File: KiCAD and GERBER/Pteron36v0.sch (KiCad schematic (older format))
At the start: 56 parts, among them J1 AudioJack4, J2 AudioJack4, J3 Conn_01x04, SW10 SW_PUSH, SW12 SW_PUSH, SW13 SW_PUSH, SW14 SW_PUSH, SW15 SW_PUSH, SW17 SW_PUSH, SW18 SW_PUSH, SW19 SW_PUSH, SW20 SW_PUSH, SW22 SW_PUSH, SW23 SW_PUSH, SW24 SW_PUSH, SW26 SW_PUSH, SW27 SW_PUSH, SW28 SW_PUSH, SW7 SW_PUSH, SW8 SW_PUSH, SW9 SW_PUSH, U1 ProMicro

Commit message: added choc and mx support in single pcb.
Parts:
- SW10, SW12, SW13, SW14, SW15, SW17, SW18, SW19, SW20, SW22, SW23, SW24, SW26, SW27, SW28, SW7, SW8, SW9: footprint Keebio-Parts:Hybrid_PCB_100H_Dual_hole -> Universal-Switch-Footprint:MX-ALPs-PG1350-FLIP
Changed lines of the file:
@@
 F 0 "SW7" H 1550 1755 50  0000 C CNN
 F 1 "SW_PUSH" H 1550 1664 50  0000 C CNN
-F 2 "Keebio-Parts:Hybrid_PCB_100H_Dual_hole" H 1550 1500 60  0001 C CNN
+F 2 "Universal-Switch-Footprint:MX-ALPs-PG1350-FLIP" H 1550 1500 60  0001 C CNN
 F 3 "" H 1550 1500 60  0000 C CNN
 	1    1550 1500
@@
 F 0 "SW8" H 1550 2405 50  0000 C CNN
 F 1 "SW_PUSH" H 1550 2314 50  0000 C CNN
-F 2 "Keebio-Parts:Hybrid_PCB_100H_Dual_hole" H 1550 2150 60  0001 C CNN
+F 2 "Universal-Switch-Footprint:MX-ALPs-PG1350-FLIP" H 1550 2150 60  0001 C CNN
 F 3 "" H 1550 2150 60  0000 C CNN
 	1    1550 2150
@@
 F 0 "SW9" H 1550 3005 50  0000 C CNN
 F 1 "SW_PUSH" H 1550 2914 50  0000 C CNN
-F 2 "Keebio-Parts:Hybrid_PCB_100H_Dual_hole" H 1550 2750 60  0001 C CNN
+F 2 "Universal-Switch-Footprint:MX-ALPs-PG1350-FLIP" H 1550 2750 60  0001 C CNN
 F 3 "" H 1550 2750 60  0000 C CNN
 	1    1550 2750
@@
 F 0 "SW12" H 2200 1755 50  0000 C CNN
 F 1 "SW_PUSH" H 2200 1664 50  0000 C CNN
-F 2 "Keebio-Parts:Hybrid_PCB_100H_Dual_hole" H 2200 1500 60  0001 C CNN
+F 2 "Universal-Switch-Footprint:MX-ALPs-PG1350-FLIP" H 2200 1500 60  0001 C CNN
 F 3 "" H 2200 1500 60  0000 C CNN
 	1    2200 1500
@@
 F 0 "SW13" H 2200 2405 50  0000 C CNN
 F 1 "SW_PUSH" H 2200 2314 50  0000 C CNN
-F 2 "Keebio-Parts:Hybrid_PCB_100H_Dual_hole" H 2200 2150 60  0001 C CNN
+F 2 "Universal-Switch-Footprint:MX-ALPs-PG1350-FLIP" H 2200 2150 60  0001 C CNN
 F 3 "" H 2200 2150 60  0000 C CNN
 	1    2200 2150
@@
 F 0 "SW14" H 2200 3005 50  0000 C CNN
 F 1 "SW_PUSH" H 2200 2914 50  0000 C CNN
-F 2 "Keebio-Parts:Hybrid_PCB_100H_Dual_hole" H 2200 2750 60  0001 C CNN
+F 2 "Universal-Switch-Footprint:MX-ALPs-PG1350-FLIP" H 2200 2750 60  0001 C CNN
 F 3 "" H 2200 2750 60  0000 C CNN
 	1    2200 2750
@@
 F 0 "SW17" H 2850 1755 50  0000 C CNN
 F 1 "SW_PUSH" H 2850 1664 50  0000 C CNN
-F 2 "Keebio-Parts:Hybrid_PCB_100H_Dual_hole" H 2850 1500 60  0001 C CNN
+F 2 "Universal-Switch-Footprint:MX-ALPs-PG1350-FLIP" H 2850 1500 60  0001 C CNN
 F 3 "" H 2850 1500 60  0000 C CNN
 	1    2850 1500
@@
 F 0 "SW22" H 3500 1755 50  0000 C CNN
 F 1 "SW_PUSH" H 3500 1664 50  0000 C CNN
-F 2 "Keebio-Parts:Hybrid_PCB_100H_Dual_hole" H 3500 1500 60  0001 C CNN
+F 2 "Universal-Switch-Footprint:MX-ALPs-PG1350-FLIP" H 3500 1500 60  0001 C CNN
 F 3 "" H 3500 1500 60  0000 C CNN
 	1    3500 1500
@@
 F 0 "SW18" H 2850 2405 50  0000 C CNN
 F 1 "SW_PUSH" H 2850 2314 50  0000 C CNN
-F 2 "Keebio-Parts:Hybrid_PCB_100H_Dual_hole" H 2850 2150 60  0001 C CNN
+F 2 "Universal-Switch-Footprint:MX-ALPs-PG1350-FLIP" H 2850 2150 60  0001 C CNN
 F 3 "" H 2850 2150 60  0000 C CNN
 	1    2850 2150
@@
 F 0 "SW19" H 2850 3005 50  0000 C CNN
 F 1 "SW_PUSH" H 2850 2914 50  0000 C CNN
-F 2 "Keebio-Parts:Hybrid_PCB_100H_Dual_hole" H 2850 2750 60  0001 C CNN
+F 2 "Universal-Switch-Footprint:MX-ALPs-PG1350-FLIP" H 2850 2750 60  0001 C CNN
 F 3 "" H 2850 2750 60  0000 C CNN
 	1    2850 2750
@@
 F 0 "SW23" H 3500 2405 50  0000 C CNN
 F 1 "SW_PUSH" H 3500 2314 50  0000 C CNN
-F 2 "Keebio-Parts:Hybrid_PCB_100H_Dual_hole" H 3500 2150 60  0001 C CNN
+F 2 "Universal-Switch-Footprint:MX-ALPs-PG1350-FLIP" H 3500 2150 60  0001 C CNN
 F 3 "" H 3500 2150 60  0000 C CNN
 	1    3500 2150
@@
 F 0 "SW24" H 3500 3005 50  0000 C CNN
 F 1 "SW_PUSH" H 3500 2914 50  0000 C CNN
-F 2 "Keebio-Parts:Hybrid_PCB_100H_Dual_hole" H 3500 2750 60  0001 C CNN
+F 2 "Universal-Switch-Footprint:MX-ALPs-PG1350-FLIP" H 3500 2750 60  0001 C CNN
 F 3 "" H 3500 2750 60  0000 C CNN
 	1    3500 2750
@@
 F 0 "SW26" H 4150 1755 50  0000 C CNN
 F 1 "SW_PUSH" H 4150 1664 50  0000 C CNN
-F 2 "Keebio-Parts:Hybrid_PCB_100H_Dual_hole" H 4150 1500 60  0001 C CNN
+F 2 "Universal-Switch-Footprint:MX-ALPs-PG1350-FLIP" H 4150 1500 60  0001 C CNN
 F 3 "" H 4150 1500 60  0000 C CNN
 	1    4150 1500
@@
 F 0 "SW27" H 4150 2405 50  0000 C CNN
 F 1 "SW_PUSH" H 4150 2314 50  0000 C CNN
-F 2 "Keebio-Parts:Hybrid_PCB_100H_Dual_hole" H 4150 2150 60  0001 C CNN
+F 2 "Universal-Switch-Footprint:MX-ALPs-PG1350-FLIP" H 4150 2150 60  0001 C CNN
 F 3 "" H 4150 2150 60  0000 C CNN
 	1    4150 2150
@@
 F 0 "SW28" H 4150 3005 50  0000 C CNN
 F 1 "SW_PUSH" H 4150 2914 50  0000 C CNN
-F 2 "Keebio-Parts:Hybrid_PCB_100H_Dual_hole" H 4150 2750 60  0001 C CNN
+F 2 "Universal-Switch-Footprint:MX-ALPs-PG1350-FLIP" H 4150 2750 60  0001 C CNN
 F 3 "" H 4150 2750 60  0000 C CNN
 	1    4150 2750
@@
 F 0 "SW10" H 1550 3605 50  0000 C CNN
 F 1 "SW_PUSH" H 1550 3514 50  0000 C CNN
-F 2 "Keebio-Parts:Hybrid_PCB_100H_Dual_hole" H 1550 3350 60  0001 C CNN
+F 2 "Universal-Switch-Footprint:MX-ALPs-PG1350-FLIP" H 1550 3350 60  0001 C CNN
 F 3 "" H 1550 3350 60  0000 C CNN
 	1    1550 3350
@@
 F 0 "SW15" H 2200 3605 50  0000 C CNN
 F 1 "SW_PUSH" H 2200 3514 50  0000 C CNN
-F 2 "Keebio-Parts:Hybrid_PCB_100H_Dual_hole" H 2200 3350 60  0001 C CNN
+F 2 "Universal-Switch-Footprint:MX-ALPs-PG1350-FLIP" H 2200 3350 60  0001 C CNN
 F 3 "" H 2200 3350 60  0000 C CNN
 	1    2200 3350
@@
 F 0 "SW20" H 2850 3605 50  0000 C CNN
 F 1 "SW_PUSH" H 2850 3514 50  0000 C CNN
-F 2 "Keebio-Parts:Hybrid_PCB_100H_Dual_hole" H 2850 3350 60  0001 C CNN
+F 2 "Universal-Switch-Footprint:MX-ALPs-PG1350-FLIP" H 2850 3350 60  0001 C CNN
 F 3 "" H 2850 3350 60  0000 C CNN
 	1    2850 3350

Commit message: merge version 1.2.0 pcb into main
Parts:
- SW10, SW12, SW13, SW14, SW15, SW17, SW18, SW19, SW20, SW22, SW23, SW24, SW26, SW27, SW28, SW7, SW8, SW9: footprint Universal-Switch-Footprint:MX-ALPs-PG1350-FLIP -> Universal-Switch-Footprint:MX-ALPs-PG1350-FLIP-fix
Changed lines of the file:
@@
 F 0 "SW7" H 1550 1755 50  0000 C CNN
 F 1 "SW_PUSH" H 1550 1664 50  0000 C CNN
-F 2 "Universal-Switch-Footprint:MX-ALPs-PG1350-FLIP" H 1550 1500 60  0001 C CNN
+F 2 "Universal-Switch-Footprint:MX-ALPs-PG1350-FLIP-fix" H 1550 1500 60  0001 C CNN
 F 3 "" H 1550 1500 60  0000 C CNN
 	1    1550 1500
@@
 F 0 "SW8" H 1550 2405 50  0000 C CNN
 F 1 "SW_PUSH" H 1550 2314 50  0000 C CNN
-F 2 "Universal-Switch-Footprint:MX-ALPs-PG1350-FLIP" H 1550 2150 60  0001 C CNN
+F 2 "Universal-Switch-Footprint:MX-ALPs-PG1350-FLIP-fix" H 1550 2150 60  0001 C CNN
 F 3 "" H 1550 2150 60  0000 C CNN
 	1    1550 2150
@@
 F 0 "SW9" H 1550 3005 50  0000 C CNN
 F 1 "SW_PUSH" H 1550 2914 50  0000 C CNN
-F 2 "Universal-Switch-Footprint:MX-ALPs-PG1350-FLIP" H 1550 2750 60  0001 C CNN
+F 2 "Universal-Switch-Footprint:MX-ALPs-PG1350-FLIP-fix" H 1550 2750 60  0001 C CNN
 F 3 "" H 1550 2750 60  0000 C CNN
 	1    1550 2750
@@
 F 0 "SW12" H 2200 1755 50  0000 C CNN
 F 1 "SW_PUSH" H 2200 1664 50  0000 C CNN
-F 2 "Universal-Switch-Footprint:MX-ALPs-PG1350-FLIP" H 2200 1500 60  0001 C CNN
+F 2 "Universal-Switch-Footprint:MX-ALPs-PG1350-FLIP-fix" H 2200 1500 60  0001 C CNN
 F 3 "" H 2200 1500 60  0000 C CNN
 	1    2200 1500
@@
 F 0 "SW13" H 2200 2405 50  0000 C CNN
 F 1 "SW_PUSH" H 2200 2314 50  0000 C CNN
-F 2 "Universal-Switch-Footprint:MX-ALPs-PG1350-FLIP" H 2200 2150 60  0001 C CNN
+F 2 "Universal-Switch-Footprint:MX-ALPs-PG1350-FLIP-fix" H 2200 2150 60  0001 C CNN
 F 3 "" H 2200 2150 60  0000 C CNN
 	1    2200 2150
@@
 F 0 "SW14" H 2200 3005 50  0000 C CNN
 F 1 "SW_PUSH" H 2200 2914 50  0000 C CNN
-F 2 "Universal-Switch-Footprint:MX-ALPs-PG1350-FLIP" H 2200 2750 60  0001 C CNN
+F 2 "Universal-Switch-Footprint:MX-ALPs-PG1350-FLIP-fix" H 2200 2750 60  0001 C CNN
 F 3 "" H 2200 2750 60  0000 C CNN
 	1    2200 2750
@@
 F 0 "SW17" H 2850 1755 50  0000 C CNN
 F 1 "SW_PUSH" H 2850 1664 50  0000 C CNN
-F 2 "Universal-Switch-Footprint:MX-ALPs-PG1350-FLIP" H 2850 1500 60  0001 C CNN
+F 2 "Universal-Switch-Footprint:MX-ALPs-PG1350-FLIP-fix" H 2850 1500 60  0001 C CNN
 F 3 "" H 2850 1500 60  0000 C CNN
 	1    2850 1500
@@
 F 0 "SW22" H 3500 1755 50  0000 C CNN
 F 1 "SW_PUSH" H 3500 1664 50  0000 C CNN
-F 2 "Universal-Switch-Footprint:MX-ALPs-PG1350-FLIP" H 3500 1500 60  0001 C CNN
+F 2 "Universal-Switch-Footprint:MX-ALPs-PG1350-FLIP-fix" H 3500 1500 60  0001 C CNN
 F 3 "" H 3500 1500 60  0000 C CNN
 	1    3500 1500
@@
 F 0 "SW18" H 2850 2405 50  0000 C CNN
 F 1 "SW_PUSH" H 2850 2314 50  0000 C CNN
-F 2 "Universal-Switch-Footprint:MX-ALPs-PG1350-FLIP" H 2850 2150 60  0001 C CNN
+F 2 "Universal-Switch-Footprint:MX-ALPs-PG1350-FLIP-fix" H 2850 2150 60  0001 C CNN
 F 3 "" H 2850 2150 60  0000 C CNN
 	1    2850 2150
@@
 F 0 "SW19" H 2850 3005 50  0000 C CNN
 F 1 "SW_PUSH" H 2850 2914 50  0000 C CNN
-F 2 "Universal-Switch-Footprint:MX-ALPs-PG1350-FLIP" H 2850 2750 60  0001 C CNN
+F 2 "Universal-Switch-Footprint:MX-ALPs-PG1350-FLIP-fix" H 2850 2750 60  0001 C CNN
 F 3 "" H 2850 2750 60  0000 C CNN
 	1    2850 2750
@@
 F 0 "SW23" H 3500 2405 50  0000 C CNN
 F 1 "SW_PUSH" H 3500 2314 50  0000 C CNN
-F 2 "Universal-Switch-Footprint:MX-ALPs-PG1350-FLIP" H 3500 2150 60  0001 C CNN
+F 2 "Universal-Switch-Footprint:MX-ALPs-PG1350-FLIP-fix" H 3500 2150 60  0001 C CNN
 F 3 "" H 3500 2150 60  0000 C CNN
 	1    3500 2150
@@
 F 0 "SW24" H 3500 3005 50  0000 C CNN
 F 1 "SW_PUSH" H 3500 2914 50  0000 C CNN
-F 2 "Universal-Switch-Footprint:MX-ALPs-PG1350-FLIP" H 3500 2750 60  0001 C CNN
+F 2 "Universal-Switch-Footprint:MX-ALPs-PG1350-FLIP-fix" H 3500 2750 60  0001 C CNN
 F 3 "" H 3500 2750 60  0000 C CNN
 	1    3500 2750
@@
 F 0 "SW26" H 4150 1755 50  0000 C CNN
 F 1 "SW_PUSH" H 4150 1664 50  0000 C CNN
-F 2 "Universal-Switch-Footprint:MX-ALPs-PG1350-FLIP" H 4150 1500 60  0001 C CNN
+F 2 "Universal-Switch-Footprint:MX-ALPs-PG1350-FLIP-fix" H 4150 1500 60  0001 C CNN
 F 3 "" H 4150 1500 60  0000 C CNN
 	1    4150 1500
@@
 F 0 "SW27" H 4150 2405 50  0000 C CNN
 F 1 "SW_PUSH" H 4150 2314 50  0000 C CNN
-F 2 "Universal-Switch-Footprint:MX-ALPs-PG1350-FLIP" H 4150 2150 60  0001 C CNN
+F 2 "Universal-Switch-Footprint:MX-ALPs-PG1350-FLIP-fix" H 4150 2150 60  0001 C CNN
 F 3 "" H 4150 2150 60  0000 C CNN
 	1    4150 2150
@@
 F 0 "SW28" H 4150 3005 50  0000 C CNN
 F 1 "SW_PUSH" H 4150 2914 50  0000 C CNN
-F 2 "Universal-Switch-Footprint:MX-ALPs-PG1350-FLIP" H 4150 2750 60  0001 C CNN
+F 2 "Universal-Switch-Footprint:MX-ALPs-PG1350-FLIP-fix" H 4150 2750 60  0001 C CNN
 F 3 "" H 4150 2750 60  0000 C CNN
 	1    4150 2750
@@
 F 0 "SW10" H 1550 3605 50  0000 C CNN
 F 1 "SW_PUSH" H 1550 3514 50  0000 C CNN
-F 2 "Universal-Switch-Footprint:MX-ALPs-PG1350-FLIP" H 1550 3350 60  0001 C CNN
+F 2 "Universal-Switch-Footprint:MX-ALPs-PG1350-FLIP-fix" H 1550 3350 60  0001 C CNN
 F 3 "" H 1550 3350 60  0000 C CNN
 	1    1550 3350
@@
 F 0 "SW15" H 2200 3605 50  0000 C CNN
 F 1 "SW_PUSH" H 2200 3514 50  0000 C CNN
-F 2 "Universal-Switch-Footprint:MX-ALPs-PG1350-FLIP" H 2200 3350 60  0001 C CNN
+F 2 "Universal-Switch-Footprint:MX-ALPs-PG1350-FLIP-fix" H 2200 3350 60  0001 C CNN
 F 3 "" H 2200 3350 60  0000 C CNN
 	1    2200 3350
@@
 F 0 "SW20" H 2850 3605 50  0000 C CNN
 F 1 "SW_PUSH" H 2850 3514 50  0000 C CNN
-F 2 "Universal-Switch-Footprint:MX-ALPs-PG1350-FLIP" H 2850 3350 60  0001 C CNN
+F 2 "Universal-Switch-Footprint:MX-ALPs-PG1350-FLIP-fix" H 2850 3350 60  0001 C CNN
 F 3 "" H 2850 3350 60  0000 C CNN
 	1    2850 3350

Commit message: use crkbd footprint for better manufacturing
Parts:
- SW10, SW12, SW13, SW14, SW15, SW17, SW18, SW19, SW20, SW22, SW23, SW24, SW26, SW27, SW28, SW7, SW8, SW9: footprint Universal-Switch-Footprint:MX-ALPs-PG1350-FLIP-fix -> User-Submitted:uni-new
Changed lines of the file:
@@
 F 0 "SW7" H 1550 1755 50  0000 C CNN
 F 1 "SW_PUSH" H 1550 1664 50  0000 C CNN
-F 2 "Universal-Switch-Footprint:MX-ALPs-PG1350-FLIP-fix" H 1550 1500 60  0001 C CNN
+F 2 "User-Submitted:uni-new" H 1550 1500 60  0001 C CNN
 F 3 "" H 1550 1500 60  0000 C CNN
 	1    1550 1500
@@
 F 0 "SW8" H 1550 2405 50  0000 C CNN
 F 1 "SW_PUSH" H 1550 2314 50  0000 C CNN
-F 2 "Universal-Switch-Footprint:MX-ALPs-PG1350-FLIP-fix" H 1550 2150 60  0001 C CNN
+F 2 "User-Submitted:uni-new" H 1550 2150 60  0001 C CNN
 F 3 "" H 1550 2150 60  0000 C CNN
 	1    1550 2150
@@
 F 0 "SW9" H 1550 3005 50  0000 C CNN
 F 1 "SW_PUSH" H 1550 2914 50  0000 C CNN
-F 2 "Universal-Switch-Footprint:MX-ALPs-PG1350-FLIP-fix" H 1550 2750 60  0001 C CNN
+F 2 "User-Submitted:uni-new" H 1550 2750 60  0001 C CNN
 F 3 "" H 1550 2750 60  0000 C CNN
 	1    1550 2750
@@
 F 0 "SW12" H 2200 1755 50  0000 C CNN
 F 1 "SW_PUSH" H 2200 1664 50  0000 C CNN
-F 2 "Universal-Switch-Footprint:MX-ALPs-PG1350-FLIP-fix" H 2200 1500 60  0001 C CNN
+F 2 "User-Submitted:uni-new" H 2200 1500 60  0001 C CNN
 F 3 "" H 2200 1500 60  0000 C CNN
 	1    2200 1500
@@
 F 0 "SW13" H 2200 2405 50  0000 C CNN
 F 1 "SW_PUSH" H 2200 2314 50  0000 C CNN
-F 2 "Universal-Switch-Footprint:MX-ALPs-PG1350-FLIP-fix" H 2200 2150 60  0001 C CNN
+F 2 "User-Submitted:uni-new" H 2200 2150 60  0001 C CNN
 F 3 "" H 2200 2150 60  0000 C CNN
 	1    2200 2150
@@
 F 0 "SW14" H 2200 3005 50  0000 C CNN
 F 1 "SW_PUSH" H 2200 2914 50  0000 C CNN
-F 2 "Universal-Switch-Footprint:MX-ALPs-PG1350-FLIP-fix" H 2200 2750 60  0001 C CNN
+F 2 "User-Submitted:uni-new" H 2200 2750 60  0001 C CNN
 F 3 "" H 2200 2750 60  0000 C CNN
 	1    2200 2750
@@
 F 0 "SW17" H 2850 1755 50  0000 C CNN
 F 1 "SW_PUSH" H 2850 1664 50  0000 C CNN
-F 2 "Universal-Switch-Footprint:MX-ALPs-PG1350-FLIP-fix" H 2850 1500 60  0001 C CNN
+F 2 "User-Submitted:uni-new" H 2850 1500 60  0001 C CNN
 F 3 "" H 2850 1500 60  0000 C CNN
 	1    2850 1500
@@
 F 0 "SW22" H 3500 1755 50  0000 C CNN
 F 1 "SW_PUSH" H 3500 1664 50  0000 C CNN
-F 2 "Universal-Switch-Footprint:MX-ALPs-PG1350-FLIP-fix" H 3500 1500 60  0001 C CNN
+F 2 "User-Submitted:uni-new" H 3500 1500 60  0001 C CNN
 F 3 "" H 3500 1500 60  0000 C CNN
 	1    3500 1500
@@
 F 0 "SW18" H 2850 2405 50  0000 C CNN
 F 1 "SW_PUSH" H 2850 2314 50  0000 C CNN
-F 2 "Universal-Switch-Footprint:MX-ALPs-PG1350-FLIP-fix" H 2850 2150 60  0001 C CNN
+F 2 "User-Submitted:uni-new" H 2850 2150 60  0001 C CNN
 F 3 "" H 2850 2150 60  0000 C CNN
 	1    2850 2150
@@
 F 0 "SW19" H 2850 3005 50  0000 C CNN
 F 1 "SW_PUSH" H 2850 2914 50  0000 C CNN
-F 2 "Universal-Switch-Footprint:MX-ALPs-PG1350-FLIP-fix" H 2850 2750 60  0001 C CNN
+F 2 "User-Submitted:uni-new" H 2850 2750 60  0001 C CNN
 F 3 "" H 2850 2750 60  0000 C CNN
 	1    2850 2750
@@
 F 0 "SW23" H 3500 2405 50  0000 C CNN
 F 1 "SW_PUSH" H 3500 2314 50  0000 C CNN
-F 2 "Universal-Switch-Footprint:MX-ALPs-PG1350-FLIP-fix" H 3500 2150 60  0001 C CNN
+F 2 "User-Submitted:uni-new" H 3500 2150 60  0001 C CNN
 F 3 "" H 3500 2150 60  0000 C CNN
 	1    3500 2150
@@
 F 0 "SW24" H 3500 3005 50  0000 C CNN
 F 1 "SW_PUSH" H 3500 2914 50  0000 C CNN
-F 2 "Universal-Switch-Footprint:MX-ALPs-PG1350-FLIP-fix" H 3500 2750 60  0001 C CNN
+F 2 "User-Submitted:uni-new" H 3500 2750 60  0001 C CNN
 F 3 "" H 3500 2750 60  0000 C CNN
 	1    3500 2750
@@
 F 0 "SW26" H 4150 1755 50  0000 C CNN
 F 1 "SW_PUSH" H 4150 1664 50  0000 C CNN
-F 2 "Universal-Switch-Footprint:MX-ALPs-PG1350-FLIP-fix" H 4150 1500 60  0001 C CNN
+F 2 "User-Submitted:uni-new" H 4150 1500 60  0001 C CNN
 F 3 "" H 4150 1500 60  0000 C CNN
 	1    4150 1500
@@
 F 0 "SW27" H 4150 2405 50  0000 C CNN
 F 1 "SW_PUSH" H 4150 2314 50  0000 C CNN
-F 2 "Universal-Switch-Footprint:MX-ALPs-PG1350-FLIP-fix" H 4150 2150 60  0001 C CNN
+F 2 "User-Submitted:uni-new" H 4150 2150 60  0001 C CNN
 F 3 "" H 4150 2150 60  0000 C CNN
 	1    4150 2150
@@
 F 0 "SW28" H 4150 3005 50  0000 C CNN
 F 1 "SW_PUSH" H 4150 2914 50  0000 C CNN
-F 2 "Universal-Switch-Footprint:MX-ALPs-PG1350-FLIP-fix" H 4150 2750 60  0001 C CNN
+F 2 "User-Submitted:uni-new" H 4150 2750 60  0001 C CNN
 F 3 "" H 4150 2750 60  0000 C CNN
 	1    4150 2750
@@
 F 0 "SW10" H 1550 3605 50  0000 C CNN
 F 1 "SW_PUSH" H 1550 3514 50  0000 C CNN
-F 2 "Universal-Switch-Footprint:MX-ALPs-PG1350-FLIP-fix" H 1550 3350 60  0001 C CNN
+F 2 "User-Submitted:uni-new" H 1550 3350 60  0001 C CNN
 F 3 "" H 1550 3350 60  0000 C CNN
 	1    1550 3350
@@
 F 0 "SW15" H 2200 3605 50  0000 C CNN
 F 1 "SW_PUSH" H 2200 3514 50  0000 C CNN
-F 2 "Universal-Switch-Footprint:MX-ALPs-PG1350-FLIP-fix" H 2200 3350 60  0001 C CNN
+F 2 "User-Submitted:uni-new" H 2200 3350 60  0001 C CNN
 F 3 "" H 2200 3350 60  0000 C CNN
 	1    2200 3350
@@
 F 0 "SW20" H 2850 3605 50  0000 C CNN
 F 1 "SW_PUSH" H 2850 3514 50  0000 C CNN
-F 2 "Universal-Switch-Footprint:MX-ALPs-PG1350-FLIP-fix" H 2850 3350 60  0001 C CNN
+F 2 "User-Submitted:uni-new" H 2850 3350 60  0001 C CNN
 F 3 "" H 2850 3350 60  0000 C CNN
 	1    2850 3350

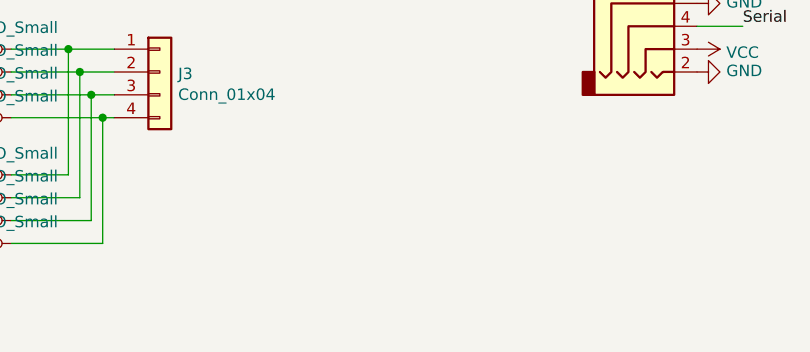
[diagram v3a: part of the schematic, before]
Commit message: final pcb
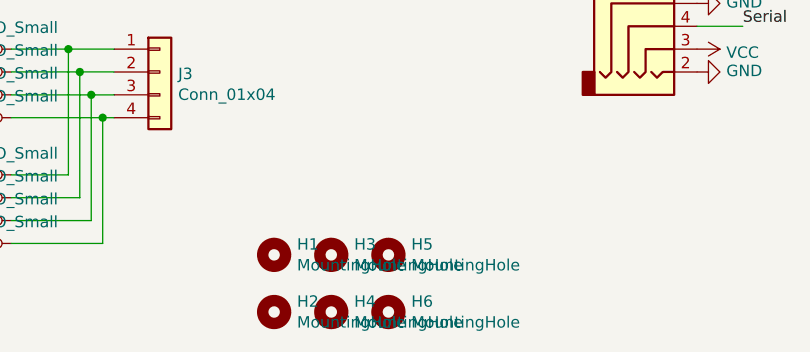
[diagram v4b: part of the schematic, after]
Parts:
- added H1, H2, H3, H4, H5, H6: MountingHole, MountingHole:MountingHole_2.2mm_M2, symbol Mechanical:MountingHole
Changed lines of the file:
@@
 NoConn ~ 8400 5250
 NoConn ~ 8400 5150
+$Comp
+L Mechanical:MountingHole H1
+U 1 1 60E75EB4
+P 5000 6600
+F 0 "H1" H 5100 6646 50  0000 L CNN
+F 1 "MountingHole" H 5100 6555 50  0000 L CNN
+F 2 "MountingHole:MountingHole_2.2mm_M2" H 5000 6600 50  0001 C CNN
+F 3 "~" H 5000 6600 50  0001 C CNN
+	1    5000 6600
+	1    0    0    -1
+$EndComp
+$Comp
+L Mechanical:MountingHole H3
+U 1 1 60E77F07
+P 5250 6600
+F 0 "H3" H 5350 6646 50  0000 L CNN
+F 1 "MountingHole" H 5350 6555 50  0000 L CNN
+F 2 "MountingHole:MountingHole_2.2mm_M2" H 5250 6600 50  0001 C CNN
+F 3 "~" H 5250 6600 50  0001 C CNN
+	1    5250 6600
+	1    0    0    -1
+$EndComp
+$Comp
+L Mechanical:MountingHole H5
+U 1 1 60E7815C
+P 5500 6600
+F 0 "H5" H 5600 6646 50  0000 L CNN
+F 1 "MountingHole" H 5600 6555 50  0000 L CNN
+F 2 "MountingHole:MountingHole_2.2mm_M2" H 5500 6600 50  0001 C CNN
+F 3 "~" H 5500 6600 50  0001 C CNN
+	1    5500 6600
+	1    0    0    -1
+$EndComp
+$Comp
+L Mechanical:MountingHole H2
+U 1 1 60E7DA87
+P 5000 6850
+F 0 "H2" H 5100 6896 50  0000 L CNN
+F 1 "MountingHole" H 5100 6805 50  0000 L CNN
+F 2 "MountingHole:MountingHole_2.2mm_M2" H 5000 6850 50  0001 C CNN
+F 3 "~" H 5000 6850 50  0001 C CNN
+	1    5000 6850
+	1    0    0    -1
+$EndComp
+$Comp
+L Mechanical:MountingHole H4
+U 1 1 60E7E592
+P 5250 6850
+F 0 "H4" H 5350 6896 50  0000 L CNN
+F 1 "MountingHole" H 5350 6805 50  0000 L CNN
+F 2 "MountingHole:MountingHole_2.2mm_M2" H 5250 6850 50  0001 C CNN
+F 3 "~" H 5250 6850 50  0001 C CNN
+	1    5250 6850
+	1    0    0    -1
+$EndComp
+$Comp
+L Mechanical:MountingHole H6
+U 1 1 60E7E974
+P 5500 6850
+F 0 "H6" H 5600 6896 50  0000 L CNN
+F 1 "MountingHole" H 5600 6805 50  0000 L CNN
+F 2 "MountingHole:MountingHole_2.2mm_M2" H 5500 6850 50  0001 C CNN
+F 3 "~" H 5500 6850 50  0001 C CNN
+	1    5500 6850
+	1    0    0    -1
+$EndComp
 $EndSCHEMATC
